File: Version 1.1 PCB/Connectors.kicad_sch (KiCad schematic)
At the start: 12 parts, among them CN3 SM06B-GHS-TB(LF)(SN), CN4 SM03B-GHS-TB(LF)(SN), J1 USB_C_Receptacle_USB2.0_14P, U10 SRV05-4-HXY, U11 SRV05-4-HXY, U13 SRV05-4-HXY, U14 SRV05-4-HXY, U7 8x Male Headers, U9 Male Headers

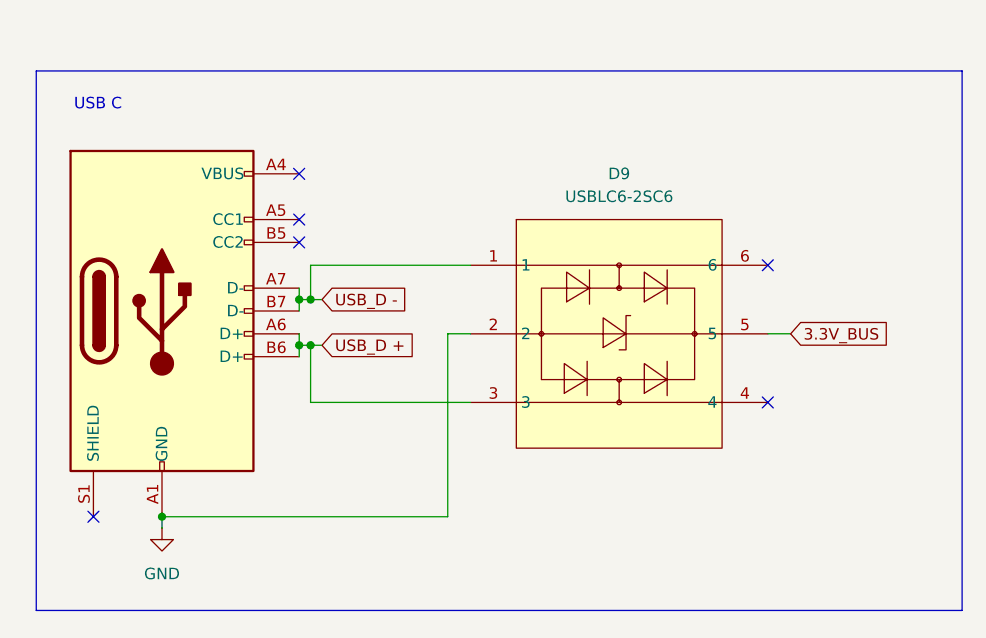
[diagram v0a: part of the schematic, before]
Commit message: began working on the routing
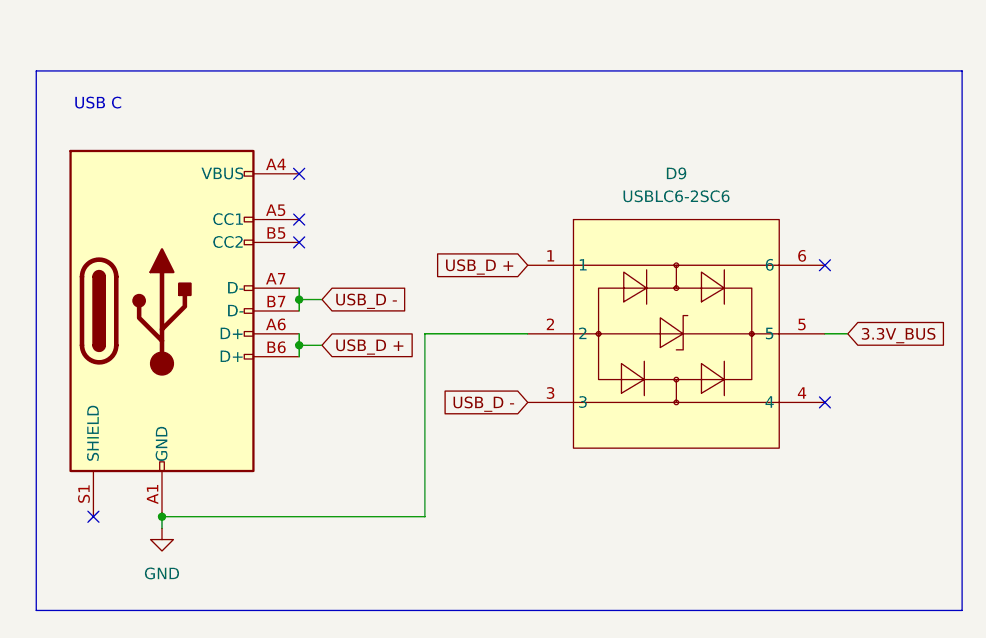
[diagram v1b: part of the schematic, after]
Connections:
- net USB_D +: now also D9.1; no longer D9.3
- net USB_D -: now also D9.3; no longer D9.1
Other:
- moved on the sheet: D9
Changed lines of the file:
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@@
-	)
-	(junction
-		(at 203.2 95.25)
-		(diameter 0)
-		(color 0 0 0 0)
 	)
 	(junction
@@
 	)
 	(junction
-		(at 203.2 100.33)
-		(diameter 0)
-		(color 0 0 0 0)
-	)
-	(junction
 		(at 77.47 120.65)
 		(diameter 0)
@@
 	)
 	(no_connect
-		(at 254 91.44)
+		(at 260.35 91.44)
 	)
 	(no_connect
@@
 	)
 	(no_connect
-		(at 254 106.68)
+		(at 260.35 106.68)
 	)
 	(no_connect
@@
 	(wire
 		(pts
-			(xy 254 99.06) (xy 256.54 99.06)
+			(xy 260.35 99.06) (xy 262.89 99.06)
 		)
 		(stroke
@@
 	(wire
 		(pts
-			(xy 203.2 100.33) (xy 203.2 106.68)
-		)
-		(stroke
-			(width 0)
-			(type default)
-		)
-	)
-	(wire
-		(pts
 			(xy 57.15 104.14) (xy 53.34 104.14)
 		)
@@
 	(wire
 		(pts
-			(xy 203.2 95.25) (xy 204.47 95.25)
-		)
-		(stroke
-			(width 0)
-			(type default)
-		)
-	)
-	(wire
-		(pts
 			(xy 77.47 115.57) (xy 77.47 118.11)
 		)
@@
 	(wire
 		(pts
-			(xy 203.2 100.33) (xy 204.47 100.33)
-		)
-		(stroke
-			(width 0)
-			(type default)
-		)
-	)
-	(wire
-		(pts
 			(xy 35.56 57.15) (xy 34.29 57.15)
 		)
@@
 	(wire
 		(pts
-			(xy 201.93 95.25) (xy 203.2 95.25)
+			(xy 201.93 95.25) (xy 204.47 95.25)
+		)
+		(stroke
+			(width 0)
+			(type default)
+		)
+	)
+	(wire
+		(pts
+			(xy 186.69 119.38) (xy 215.9 119.38)
 		)
 		(stroke
@@
 	(wire
 		(pts
-			(xy 203.2 106.68) (xy 220.98 106.68)
-		)
-		(stroke
-			(width 0)
-			(type default)
-		)
-	)
-	(wire
-		(pts
 			(xy 201.93 93.98) (xy 201.93 95.25)
 		)
@@
 	(wire
 		(pts
-			(xy 203.2 91.44) (xy 220.98 91.44)
-		)
-		(stroke
-			(width 0)
-			(type default)
-		)
-	)
-	(wire
-		(pts
 			(xy 186.69 120.65) (xy 186.69 119.38)
 		)
@@
 	(wire
 		(pts
-			(xy 218.44 99.06) (xy 220.98 99.06)
+			(xy 215.9 99.06) (xy 227.33 99.06)
 		)
 		(stroke
@@
 	(wire
 		(pts
-			(xy 218.44 99.06) (xy 218.44 119.38)
-		)
-		(stroke
-			(width 0)
-			(type default)
-		)
-	)
-	(wire
-		(pts
-			(xy 218.44 119.38) (xy 186.69 119.38)
-		)
-		(stroke
-			(width 0)
-			(type default)
-		)
-	)
-	(wire
-		(pts
-			(xy 203.2 95.25) (xy 203.2 91.44)
+			(xy 215.9 99.06) (xy 215.9 119.38)
 		)
 		(stroke
@@
 	(wire
 		(pts
-			(xy 201.93 100.33) (xy 203.2 100.33)
+			(xy 201.93 100.33) (xy 204.47 100.33)
 		)
 		(stroke
@@
 		)
 	)
+	(global_label "USB_D +"
+		(shape input)
+		(at 227.33 91.44 180)
+		(fields_autoplaced yes)
+		(effects
+			(font
+				(size 1.27 1.27)
+			)
+			(justify right)
+		)
+		(property "Intersheetrefs" "${INTERSHEET_REFS}"
+			(at 215.7572 91.44 0)
+			(effects
+				(font
+					(size 1.27 1.27)
+				)
+				(justify right)
+				(hide yes)
+			)
+		)
+	)
 	(global_label "ENCODER_CLK"
 		(shape input)
@@
 	(global_label "3.3V_BUS"
 		(shape input)
-		(at 256.54 99.06 0)
-		(fields_autoplaced yes)
-		(effects
-			(font
-				(size 1.27 1.27)
-			)
-			(justify left)
-		)
-		(property "Intersheetrefs" "${INTERSHEET_REFS}"
-			(at 268.4152 99.06 0)
+		(at 262.89 99.06 0)
+		(fields_autoplaced yes)
+		(effects
+			(font
+				(size 1.27 1.27)
+			)
+			(justify left)
+		)
+		(property "Intersheetrefs" "${INTERSHEET_REFS}"
+			(at 274.7652 99.06 0)
 			(effects
 				(font
@@
 		(property "Intersheetrefs" "${INTERSHEET_REFS}"
 			(at 105.6905 116.84 0)
+			(effects
+				(font
+					(size 1.27 1.27)
+				)
+				(justify right)
+				(hide yes)
+			)
+		)
+	)
+	(global_label "USB_D -"
+		(shape input)
+		(at 227.33 106.68 180)
+		(fields_autoplaced yes)
+		(effects
+			(font
+				(size 1.27 1.27)
+			)
+			(justify right)
+		)
+		(property "Intersheetrefs" "${INTERSHEET_REFS}"
+			(at 215.7572 106.68 0)
 			(effects
 				(font
@@
 	(symbol
 		(lib_id "easyeda2kicad:USBLC6-2SC6")
-		(at 237.49 99.06 0)
+		(at 243.84 99.06 0)
 		(unit 1)
 		(exclude_from_sim no)
@@
 		(fields_autoplaced yes)
 		(property "Reference" "D9"
-			(at 237.49 81.28 0)
+			(at 243.84 81.28 0)
 			(effects
 				(font
@@
 		)
 		(property "Value" "USBLC6-2SC6"
-			(at 237.49 83.82 0)
+			(at 243.84 83.82 0)
 			(effects
 				(font
@@
 		)
 		(property "Footprint" "easyeda2kicad:SOT-23-6_L2.9-W1.6-P0.95-LS2.8-BL"
-			(at 237.49 114.3 0)
+			(at 243.84 114.3 0)
 			(effects
 				(font
@@
 		)
 		(property "Datasheet" "https://lcsc.com/product-detail/Diodes-ESD_STMicroelectronics_USBLC6-2SC6_USBLC6-2SC6_C7519.html"
-			(at 237.49 116.84 0)
+			(at 243.84 116.84 0)
 			(effects
 				(font
@@
 		)
 		(property "Description" ""
-			(at 237.49 99.06 0)
+			(at 243.84 99.06 0)
 			(effects
 				(font
@@
 		)
 		(property "LCSC Part" "C7519"
-			(at 237.49 119.38 0)
+			(at 243.84 119.38 0)
 			(effects
 				(font
@@
 		)
 		(property "Sim.Device" ""
-			(at 237.49 99.06 0)
+			(at 243.84 99.06 0)
 			(effects
 				(font
@@
 		)
 		(property "Sim.Type" ""
-			(at 237.49 99.06 0)
-			(effects
-				(font
+			(at 243.84 99.06 0)
+			(effects
+				(font
